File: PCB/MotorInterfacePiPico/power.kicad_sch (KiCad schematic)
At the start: 19 parts, among them U2 OPA4197, U3 LM7810, U4 LM79L05

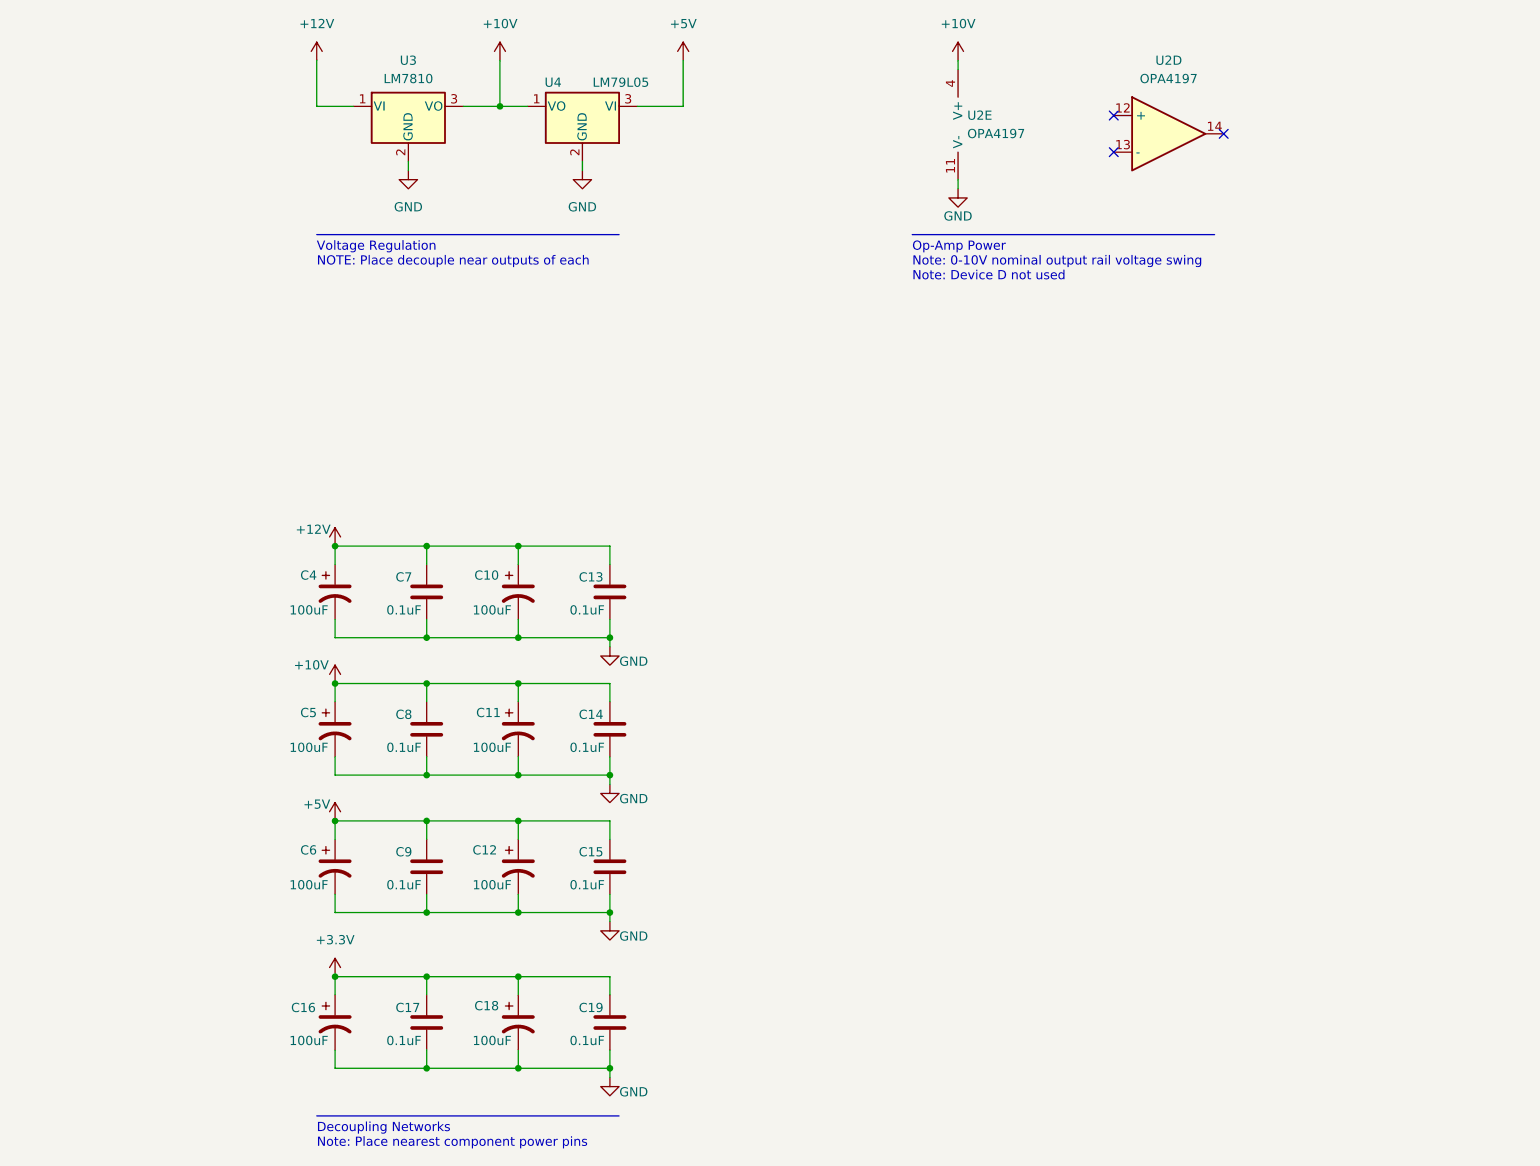
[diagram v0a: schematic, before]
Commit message: add MotorInterfacePiPico
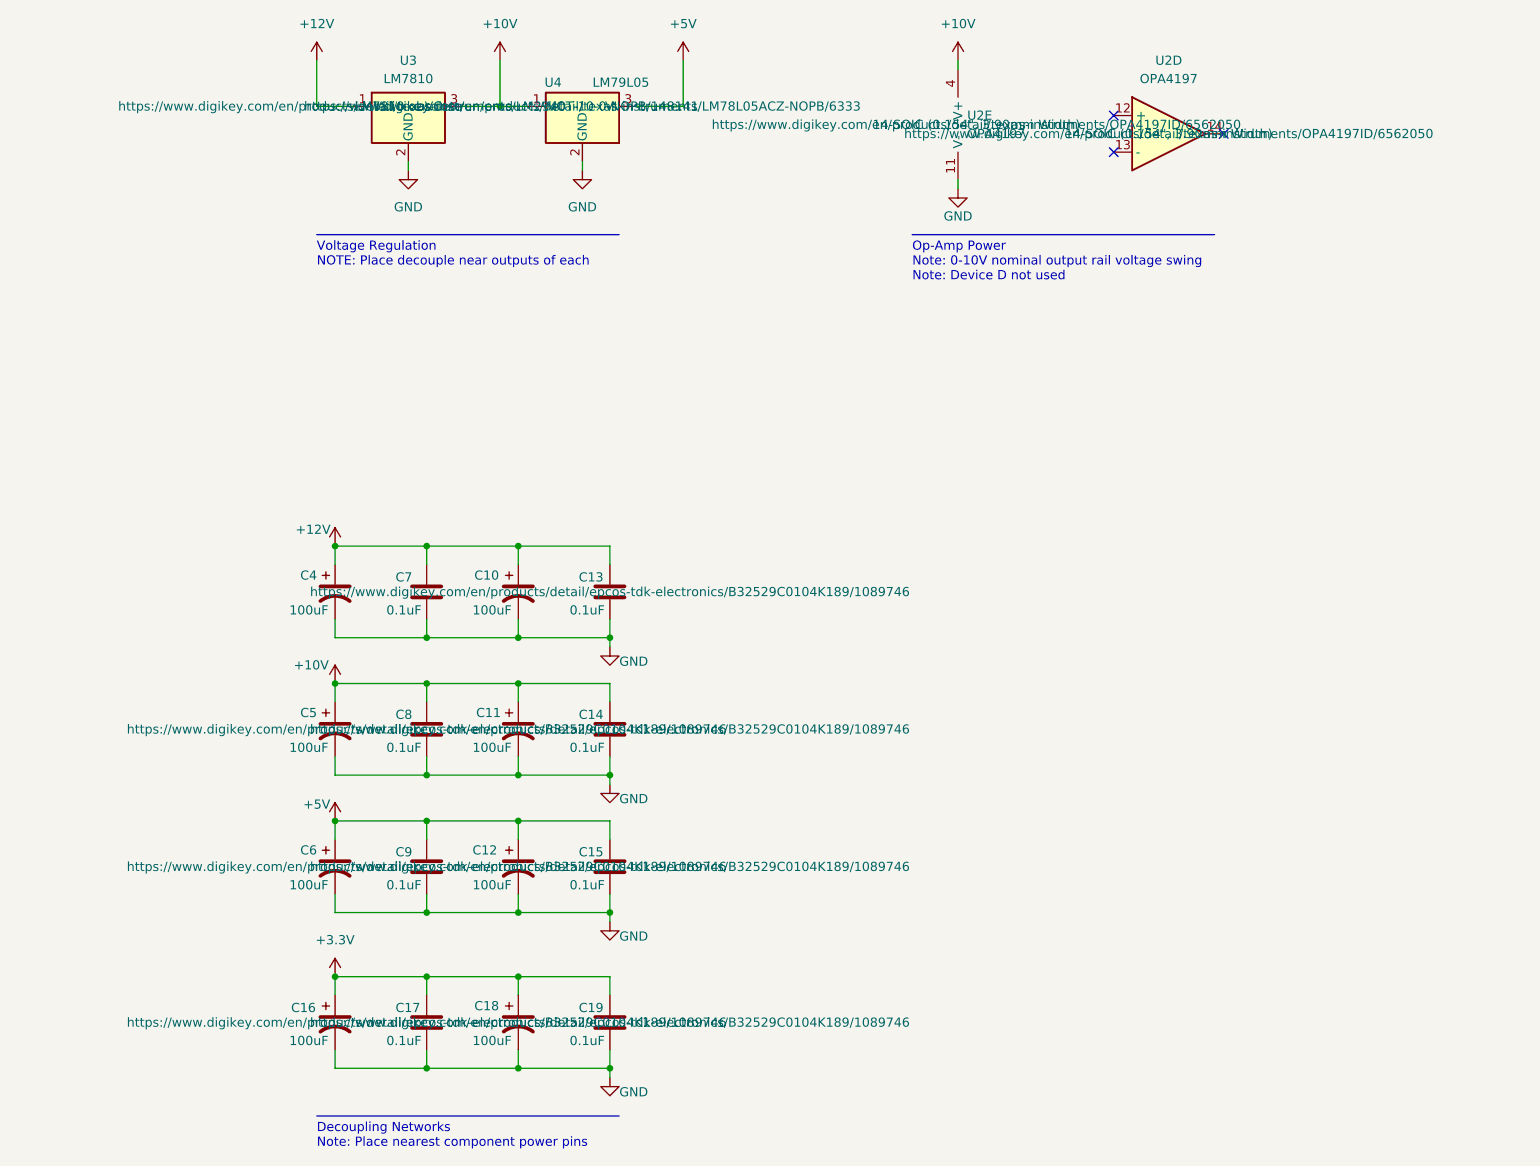
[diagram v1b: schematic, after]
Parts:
- C13, C14, C15, C17, C19, C8, C9: digikey (none) -> https://www.digikey.com/en/products/detail/epcos-tdk-electr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
- U2: Notes (none) -> 14-SOIC (0.154", 3.90mm Width); digikey (none) -> https://www.digikey.com/en/products/detail/texas-instrument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
- U3: Notes (none) -> LM7810 obsolete; digikey (none) -> https://www.digikey.com/en/products/detail/texas-instrument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
- U4: digikey (none) -> https://www.digikey.com/en/products/detail/texas-instrument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
